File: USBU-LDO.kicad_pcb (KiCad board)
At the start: 2 copper layers, 20 x 13 mm, 7 parts, among them J1 USB_B_Micro, J2 Conn_01x05_Pin, U1 AMS1117-3.3

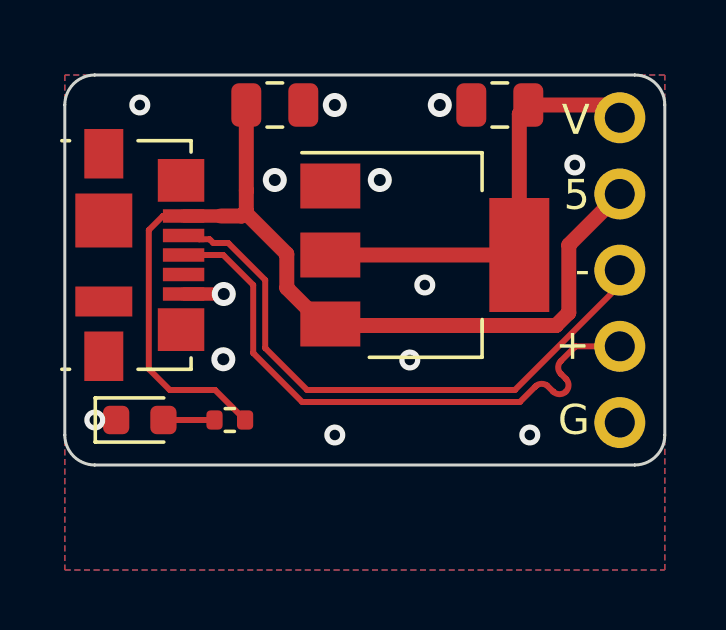
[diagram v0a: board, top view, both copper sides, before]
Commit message: Generated CAM files
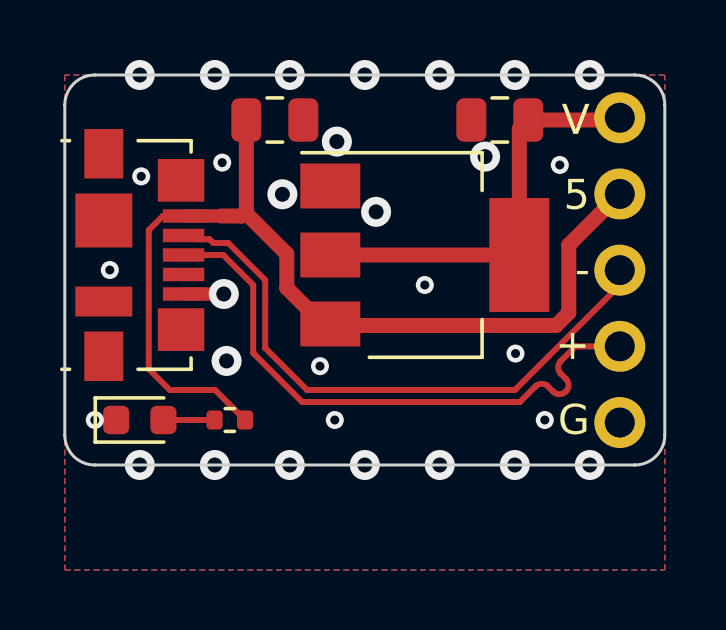
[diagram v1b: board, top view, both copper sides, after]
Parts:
- moved C1 0.50 mm to (157.0, 95.0)
- moved C2 0.50 mm to (164.5, 95.0)
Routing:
- net VCC: track 14.7 -> 14.1 mm
- net VBUS: track 33.5 -> 33.0 mm
- net GND: vias 13 -> 30
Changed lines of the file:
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@@
   (net 8 "/D+")
   (footprint "Capacitor_SMD:C_0805_2012Metric" (layer "F.Cu")
-    (at 164.5 94.5 180)
+    (at 164.5 95 180)
     (descr "Capacitor SMD 0805 (2012 Metric), square (rectangular) end terminal, IPC_7351 nominal, (Body size source: IPC-SM-782 page 76, https://www.pcb-3d.com/wordpress/wp-content/uploads/ipc-sm-782a_amendment_1_and_2.pdf, https://docs.google.com/spreadsheets/d/1BsfQQcO9C6DZCsRaXUlFlo91Tg2WpOkGARC1WS5S8t0/edit?usp=sharing), generated with kicad-footprint-generator")
     (tags "capacitor")
@@
   )
   (footprint "Capacitor_SMD:C_0805_2012Metric" (layer "F.Cu")
-    (at 157 94.5)
+    (at 157 95)
     (descr "Capacitor SMD 0805 (2012 Metric), square (rectangular) end terminal, IPC_7351 nominal, (Body size source: IPC-SM-782 page 76, https://www.pcb-3d.com/wordpress/wp-content/uploads/ipc-sm-782a_amendment_1_and_2.pdf, https://docs.google.com/spreadsheets/d/1BsfQQcO9C6DZCsRaXUlFlo91Tg2WpOkGARC1WS5S8t0/edit?usp=sharing), generated with kicad-footprint-generator")
     (tags "capacitor")
@@
   (segment (start 166.80029 101.424392) (end 166.80029 99.16471) (width 0.5) (layer "F.Cu") (net 1))
   (segment (start 156.05 98.115293) (end 156.05 98.05) (width 0.5) (layer "F.Cu") (net 1))
-  (segment (start 156.05 98.05) (end 156.05 97.35) (width 0.5) (layer "F.Cu") (net 1))
   (segment (start 166.374682 101.85) (end 166.80029 101.424392) (width 0.5) (layer "F.Cu") (net 1))
   (segment (start 158.85 101.8) (end 158.6 101.8) (width 0.5) (layer "F.Cu") (net 1))
@@
   (segment (start 157.4 99.465293) (end 156.05 98.115293) (width 0.5) (layer "F.Cu") (net 1))
   (segment (start 156.05 98.05) (end 155.9 98.2) (width 0.5) (layer "F.Cu") (net 1))
-  (segment (start 156.05 94.5) (end 156.05 97.35) (width 0.5) (layer "F.Cu") (net 1))
   (segment (start 158.85 101.8) (end 158.9 101.85) (width 0.5) (layer "F.Cu") (net 1))
+  (segment (start 156.05 95) (end 156.05 98.05) (width 0.5) (layer "F.Cu") (net 1))
   (segment (start 155.9 98.2) (end 155.2 98.2) (width 0.5) (layer "F.Cu") (net 1))
   (segment (start 152.8 103.3) (end 152.8 98.67) (width 0.2) (layer "F.Cu") (net 1))
@@
   (segment (start 153.27 98.2) (end 153.96 98.2) (width 0.2) (layer "F.Cu") (net 1))
   (segment (start 155.3 100.8) (end 153.96 100.8) (width 0.45) (layer "F.Cu") (net 2))
-  (via (at 162 100.5) (size 0.7) (drill 0.35) (layers "F.Cu" "B.Cu") (free) (net 2))
-  (via (at 155.3 100.8) (size 0.8) (drill 0.4) (layers "F.Cu" "B.Cu") (net 2))
-  (via (at 159 105.5) (size 0.7) (drill 0.35) (layers "F.Cu" "B.Cu") (free) (net 2))
-  (via (at 159 94.5) (size 0.8) (drill 0.4) (layers "F.Cu" "B.Cu") (free) (net 2))
-  (via (at 152.5 94.5) (size 0.7) (drill 0.35) (layers "F.Cu" "B.Cu") (free) (net 2))
-  (via (at 160.5 97) (size 0.8) (drill 0.4) (layers "F.Cu" "B.Cu") (free) (net 2))
-  (via (at 157 97) (size 0.8) (drill 0.4) (layers "F.Cu" "B.Cu") (free) (net 2))
-  (via (at 161.5 103) (size 0.7) (drill 0.35) (layers "F.Cu" "B.Cu") (free) (net 2))
-  (via (at 151 105) (size 0.7) (drill 0.35) (layers "F.Cu" "B.Cu") (free) (net 2))
-  (via (at 167 96.5) (size 0.7) (drill 0.35) (layers "F.Cu" "B.Cu") (free) (net 2))
-  (via (at 155.283997 102.975318) (size 0.8) (drill 0.4) (layers "F.Cu" "B.Cu") (free) (net 2))
-  (via (at 165.5 105.5) (size 0.7) (drill 0.35) (layers "F.Cu" "B.Cu") (free) (net 2))
-  (via (at 162.5 94.5) (size 0.8) (drill 0.4) (layers "F.Cu" "B.Cu") (free) (net 2))
+  (via (at 160 106.5) (size 1) (drill 0.5) (layers "F.Cu" "B.Cu") (free) (net 2))
+  (via (at 155 93.5) (size 1) (drill 0.5) (layers "F.Cu" "B.Cu") (free) (net 2))
+  (via (at 155.246645 96.420404) (size 0.6) (drill 0.3) (layers "F.Cu" "B.Cu") (free) (net 2))
+  (via (at 151.5 100) (size 0.6) (drill 0.3) (layers "F.Cu" "B.Cu") (free) (net 2))
+  (via (at 159 105) (size 0.6) (drill 0.3) (layers "F.Cu" "B.Cu") (free) (net 2))
+  (via (at 166.5 96.5) (size 0.6) (drill 0.3) (layers "F.Cu" "B.Cu") (free) (net 2))
+  (via (at 165 93.5) (size 1) (drill 0.5) (layers "F.Cu" "B.Cu") (free) (net 2))
+  (via (at 152.5 93.5) (size 1) (drill 0.5) (layers "F.Cu" "B.Cu") (free) (net 2))
+  (via (at 155.3 100.8) (size 1) (drill 0.5) (layers "F.Cu" "B.Cu") (net 2))
+  (via (at 162.5 106.5) (size 1) (drill 0.5) (layers "F.Cu" "B.Cu") (free) (net 2))
+  (via (at 167.5 93.5) (size 1) (drill 0.5) (layers "F.Cu" "B.Cu") (free) (net 2))
+  (via (at 152.547712 96.878713) (size 0.6) (drill 0.3) (layers "F.Cu" "B.Cu") (free) (net 2))
+  (via (at 157.5 93.5) (size 1) (drill 0.5) (layers "F.Cu" "B.Cu") (free) (net 2))
+  (via (at 167.5 106.5) (size 1) (drill 0.5) (layers "F.Cu" "B.Cu") (free) (net 2))
+  (via (at 165 106.5) (size 1) (drill 0.5) (layers "F.Cu" "B.Cu") (free) (net 2))
+  (via (at 160.376419 98.061646) (size 1) (drill 0.5) (layers "F.Cu" "B.Cu") (free) (net 2))
+  (via (at 155.392495 103.031272) (size 1) (drill 0.5) (layers "F.Cu" "B.Cu") (free) (net 2))
+  (via (at 165.023912 102.785812) (size 0.6) (drill 0.3) (layers "F.Cu" "B.Cu") (free) (net 2))
+  (via (at 157.253125 97.476029) (size 1) (drill 0.5) (layers "F.Cu" "B.Cu") (free) (net 2))
+  (via (at 155 106.5) (size 1) (drill 0.5) (layers "F.Cu" "B.Cu") (free) (net 2))
+  (via (at 166 105) (size 0.6) (drill 0.3) (layers "F.Cu" "B.Cu") (free) (net 2))
+  (via (at 159.069388 95.719176) (size 1) (drill 0.5) (layers "F.Cu" "B.Cu") (free) (net 2))
+  (via (at 158.505734 103.205929) (size 0.6) (drill 0.3) (layers "F.Cu" "B.Cu") (free) (net 2))
+  (via (at 152.5 106.5) (size 1) (drill 0.5) (layers "F.Cu" "B.Cu") (free) (net 2))
+  (via (at 162.5 93.5) (size 1) (drill 0.5) (layers "F.Cu" "B.Cu") (free) (net 2))
+  (via (at 160 93.5) (size 1) (drill 0.5) (layers "F.Cu" "B.Cu") (free) (net 2))
+  (via (at 162 100.5) (size 0.6) (drill 0.3) (layers "F.Cu" "B.Cu") (free) (net 2))
+  (via (at 151 105) (size 0.6) (drill 0.3) (layers "F.Cu" "B.Cu") (free) (net 2))
+  (via (at 157.5 106.5) (size 1) (drill 0.5) (layers "F.Cu" "B.Cu") (free) (net 2))
+  (via (at 164.009232 96.219922) (size 1) (drill 0.5) (layers "F.Cu" "B.Cu") (free) (net 2))
+  (segment (start 165.15 95.3) (end 165.45 95) (width 0.5) (layer "F.Cu") (net 3))
   (segment (start 158.85 99.8) (end 158.9 99.85) (width 0.5) (layer "F.Cu") (net 3))
   (segment (start 158.85 99.5) (end 165.15 99.5) (width 0.5) (layer "F.Cu") (net 3))
-  (segment (start 165.45 94.5) (end 168.075 94.5) (width 0.5) (layer "F.Cu") (net 3))
-  (segment (start 165.15 94.8) (end 165.45 94.5) (width 0.5) (layer "F.Cu") (net 3))
-  (segment (start 168.075 94.5) (end 168.5 94.925) (width 0.5) (layer "F.Cu") (net 3))
-  (segment (start 165.15 99.5) (end 165.15 94.8) (width 0.5) (layer "F.Cu") (net 3))
+  (segment (start 168.425 95) (end 168.5 94.925) (width 0.5) (layer "F.Cu") (net 3))
+  (segment (start 165.45 95) (end 168.425 95) (width 0.5) (layer "F.Cu") (net 3))
+  (segment (start 165.15 99.5) (end 165.15 95.3) (width 0.5) (layer "F.Cu") (net 3))
   (segment (start 153.2875 105) (end 154.99 105) (width 0.2) (layer "F.Cu") (net 4))
   (segment (start 155.446279 99.1) (end 156.680593 100.334315) (width 0.2) (layer "F.Cu") (net 7))
